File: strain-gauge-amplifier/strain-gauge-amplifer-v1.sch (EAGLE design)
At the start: 19 parts, among them IC2 INA125U, Q1 PMV45EN

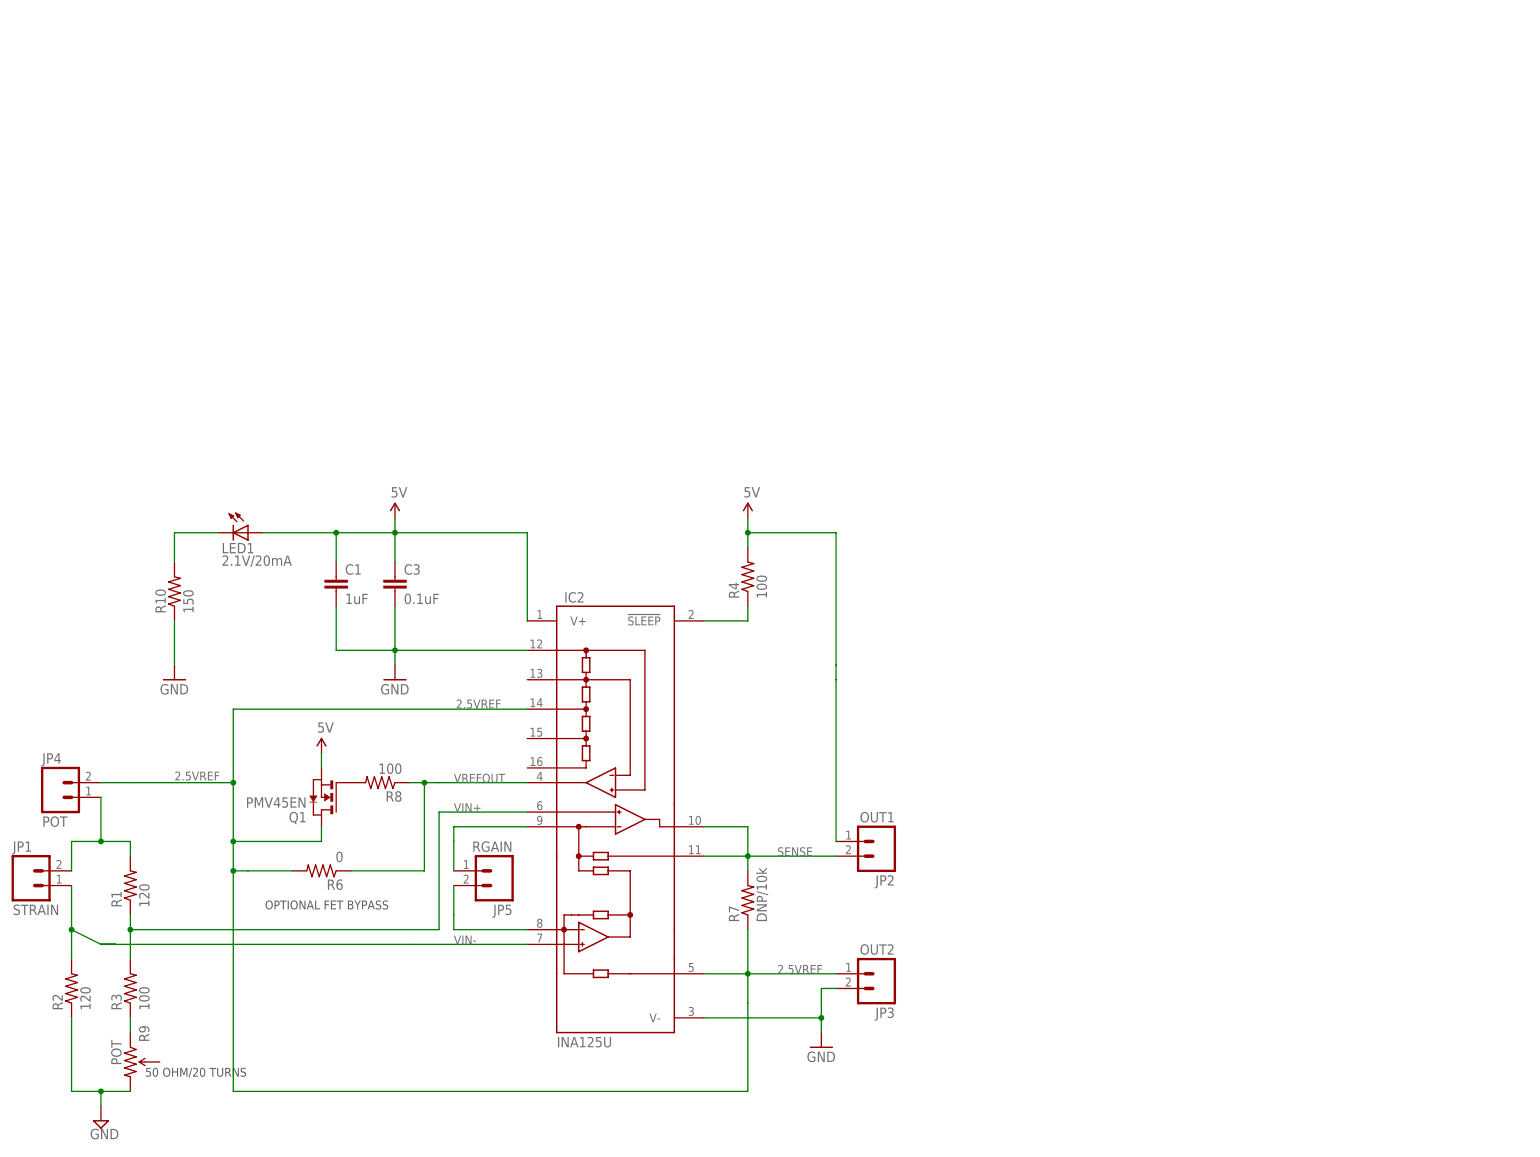
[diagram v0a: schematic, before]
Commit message: Cleaned up schematic, fixed a minor errors, ready for layout!
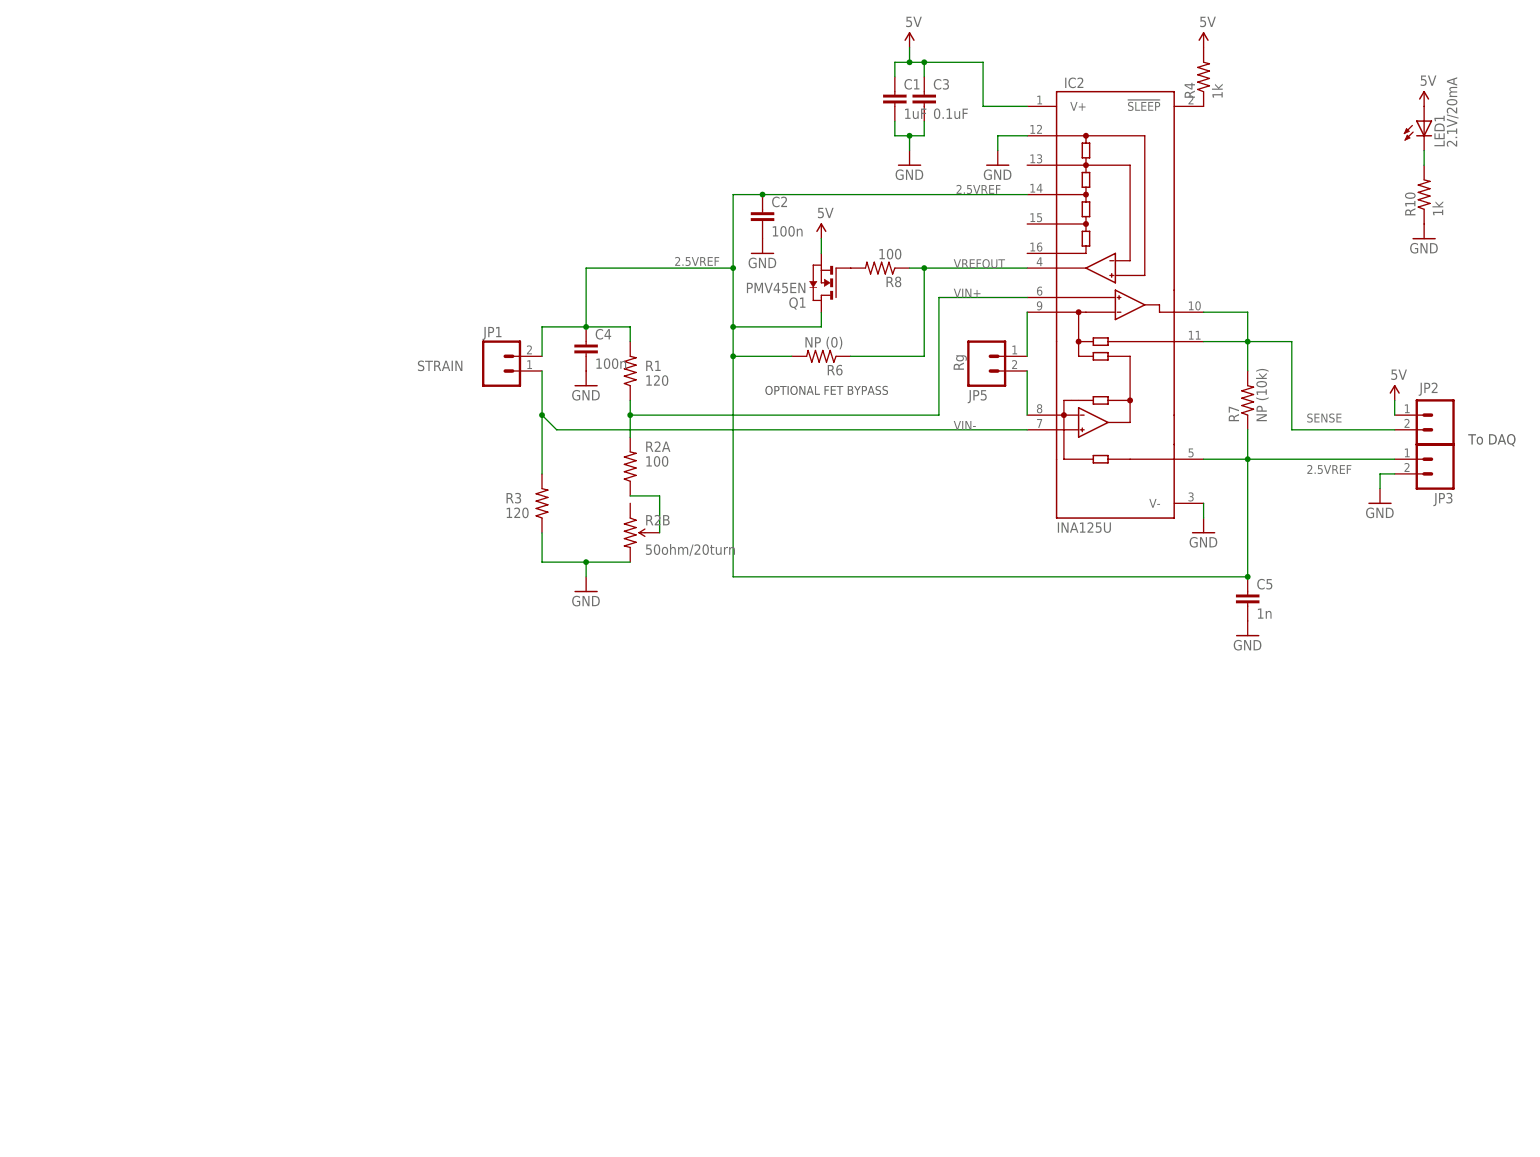
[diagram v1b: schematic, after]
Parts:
- removed JP4: POT, SparkFun-Connectors:M025MM
- removed R2: 120, rcl_custom:R-US_0805-C-NOSILK
- removed R9: POT, SparkFun-Electromechanical:TRIMPOTTRIMPOT-5MM
- added C2, C4: 100n, rcl_custom:C-EU0805-C-NOSILK
- added C5: 1n, rcl_custom:C-EU0805-C-NOSILK
- added R2A: 100, rcl_custom:R-US_0805-C-NOSILK
- added R2B: 50ohm/20turn, SparkFun-Electromechanical:TRIMPOTTRIMPOT-5MM
- JP2: value OUT1 -> (none)
- JP3: value OUT2 -> (none)
- JP5: value RGAIN -> Rg
- R10: value 150 -> 1k
- R3: value 100 -> 120
- R4: value 100 -> 1k
- R6: value 0 -> NP (0)
- R7: value DNP/10k -> NP (10k)
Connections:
- removed net N$7: R3.1, R9.CCW
- net 2.5VREF: now also C2.1, C4.1, C5.1, JP1.2, R1.2; no longer JP4.2
- net GND: now also C2.2, C4.2, C5.2, R2B.CW, R3.1; no longer R2.1, R9.CW
- net N$1: now also R2A.1, R2B.WIPER; no longer JP1.2, JP4.1, R1.2
- net VIN+: now also R2A.2; no longer R3.2
- net VIN-: now also R3.2; no longer R2.2
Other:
- note added: "To DAQ"
- note removed: "50 OHM/20 TURNS"
- moved on the sheet: C1, C3, IC2, JP1, JP2, JP3, JP5, LED1, Q1, R1, R10, R3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
